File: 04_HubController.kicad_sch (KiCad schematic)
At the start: 1 part, among them U13 CYUSB3304-68LTXx

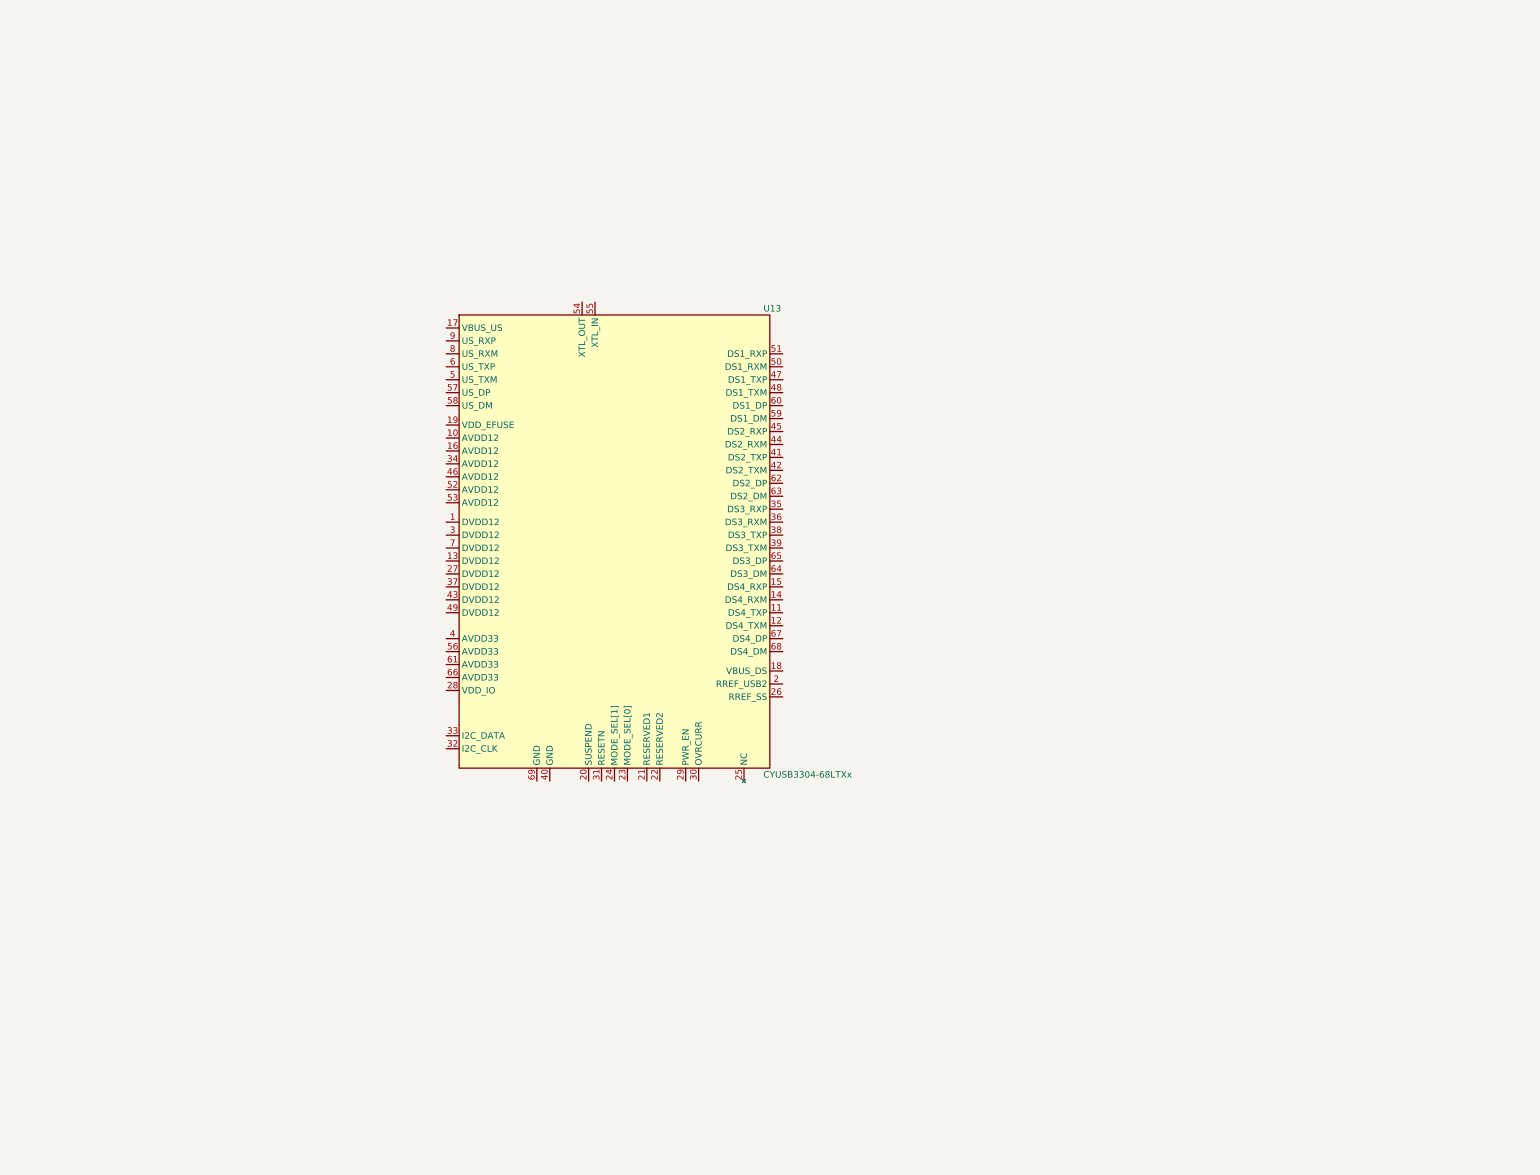
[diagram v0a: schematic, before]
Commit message: WIP hub and DFP
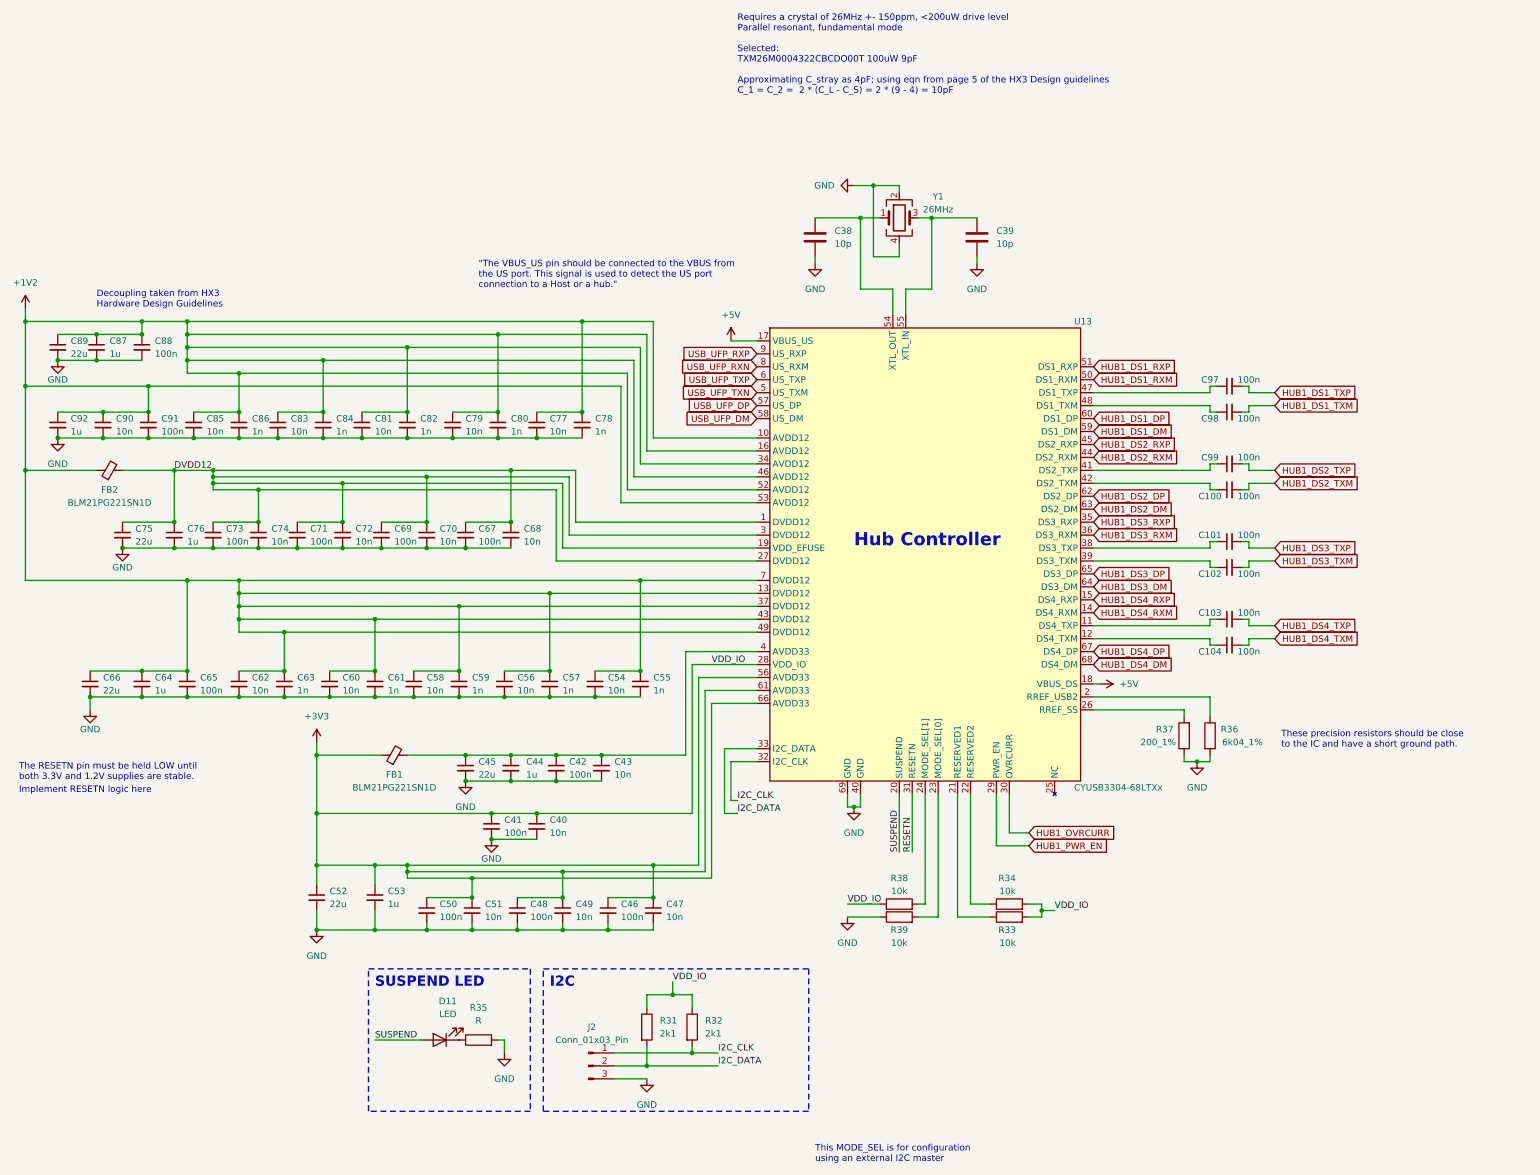
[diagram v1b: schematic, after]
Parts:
- added C100, C101, C102, C103, C104, C41, C42, C46, C48, C50, C65, C67, C69, C71, C73, C88, C91, C97, C98, C99: 100n, symbol Device:C_Small
- added C38, C39: 10p, symbol Device:C
- added C40, C43, C47, C49, C51, C54, C56, C58, C60, C62, C68, C70, C72, C74, C77, C79, C81, C83, C85, C90: 10n, symbol Device:C_Small
- added C44, C53, C64, C76, C87, C92: 1u, symbol Device:C_Small
- added C45, C52, C66, C75, C89: 22u, symbol Device:C_Small
- added C55, C57, C59, C61, C63, C78, C80, C82, C84, C86: 1n, symbol Device:C_Small
- added D11: LED, symbol Device:LED
- added FB1, FB2: BLM21PG221SN1D, symbol Device:FerriteBead_Small
- added J2: Conn_01x03_Pin, symbol Connector:Conn_01x03_Pin
- added R31, R32: 2k1, symbol Device:R
- added R33, R34, R38, R39: 10k, symbol Device:R
- added R35: R, symbol Device:R
- added R36: 6k04_1%, symbol Device:R
- added R37: 200_1%, symbol Device:R
- added Y1: 26MHz, symbol Device:Crystal_GND24
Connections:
- net DVDD12: now reaches U13.1 (DVDD12)
- net DVDD12: now also U13.19 (VDD_EFUSE), U13.27 (DVDD12), U13.3 (DVDD12), C67.1, C68.1, C69.1, C70.1, C71.1, C72.1, C73.1, C74.1, C75.1, C76.1, FB2.2
- net +1V2: now reaches U13.10 (AVDD12)
- net +1V2: now also U13.13 (DVDD12), U13.16 (AVDD12), U13.34 (AVDD12), U13.37 (DVDD12), U13.43 (DVDD12), U13.46 (AVDD12), U13.49 (DVDD12), U13.52 (AVDD12), U13.53 (AVDD12), U13.7 (DVDD12), C54.1, C55.1, C56.1, C57.1, C58.1, C59.1, C60.1, C61.1, C62.1, C63.1, C64.1, C65.1, C66.1, C77.1, C78.1, C79.1, C80.1, C81.1, C82.1, C83.1, C84.1, C85.1, C86.1, C87.1, C88.1, C89.1, C90.1, C91.1, C92.1, FB2.1
- net at U13.11 (DS4_TXP): now also C103.1
- net at U13.12 (DS4_TXM): now also C104.1
- net HUB1_DS4_RXM: now reaches U13.14 (DS4_RXM)
- net HUB1_DS4_RXP: now reaches U13.15 (DS4_RXP)
- net +5V: now reaches U13.17 (VBUS_US)
- net +5V: now also U13.18 (VBUS_DS)
- net at U13.2 (RREF_USB2): now also R36.1
- net SUSPEND: now reaches U13.20 (SUSPEND)
- net SUSPEND: now also D11.2 (A)
- net at U13.21 (RESERVED1): now also R33.1
- net at U13.22 (RESERVED2): now also R34.1
- net at U13.23 (MODE_SEL[0]): now also R39.2
- net at U13.24 (MODE_SEL[1]): now also R38.2
- net at U13.26 (RREF_SS): now also R37.2
- net +3V3: now reaches U13.28 (VDD_IO)
- net +3V3: now also U13.56 (AVDD33), U13.61 (AVDD33), U13.66 (AVDD33), C40.1, C41.1, C46.1, C47.1, C48.1, C49.1, C50.1, C51.1, C52.1, C53.1, FB1.1, R31.1, R32.1, R33.2, R34.2, R38.1
- net HUB1_PWR_EN: now reaches U13.29 (PWR_EN)
- net HUB1_OVRCURR: now reaches U13.30 (OVRCURR)
- net RESETN: now reaches U13.31 (RESETN)
- net I2C_CLK: now reaches U13.32 (I2C_CLK)
- net I2C_CLK: now also J2.1 (Pin_1), R32.2
- net I2C_DATA: now reaches U13.33 (I2C_DATA)
- net I2C_DATA: now also J2.2 (Pin_2), R31.2
- net HUB1_DS3_RXP: now reaches U13.35 (DS3_RXP)
- net HUB1_DS3_RXM: now reaches U13.36 (DS3_RXM)
- net at U13.38 (DS3_TXP): now also C101.1
- net at U13.39 (DS3_TXM): now also C102.1
- net at U13.4 (AVDD33): now also C42.1, C43.1, C44.1, C45.1, FB1.2
- net GND: now reaches U13.40 (GND)
- net GND: now also U13.69 (GND), C38.2, C39.2, C40.2, C41.2, C42.2, C43.2, C44.2, C45.2, C46.2, C47.2, C48.2, C49.2, C50.2, C51.2, C52.2, C53.2, C54.2, C55.2, C56.2, C57.2, C58.2, C59.2, C60.2, C61.2, C62.2, C63.2, C64.2, C65.2, C66.2, C67.2, C68.2, C69.2, C70.2, C71.2, C72.2, C73.2, C74.2, C75.2, C76.2, C77.2, C78.2, C79.2, C80.2, C81.2, C82.2, C83.2, C84.2, C85.2, C86.2, C87.2, C88.2, C89.2, C90.2, C91.2, C92.2, J2.3 (Pin_3), R35.2, R36.2, R37.1, R39.1, Y1.2, Y1.4
- net at U13.41 (DS2_TXP): now also C99.1
- net at U13.42 (DS2_TXM): now also C100.1
- net HUB1_DS2_RXM: now reaches U13.44 (DS2_RXM)
- net HUB1_DS2_RXP: now reaches U13.45 (DS2_RXP)
- net at U13.47 (DS1_TXP): now also C97.1
- net at U13.48 (DS1_TXM): now also C98.1
- net USB_UFP_TXN: now reaches U13.5 (US_TXM)
- net HUB1_DS1_RXM: now reaches U13.50 (DS1_RXM)
- net HUB1_DS1_RXP: now reaches U13.51 (DS1_RXP)
- net at U13.54 (XTL_OUT): now also C38.1, Y1.1
- net at U13.55 (XTL_IN): now also C39.1, Y1.3
- net USB_UFP_DP: now reaches U13.57 (US_DP)
- net USB_UFP_DM: now reaches U13.58 (US_DM)
- net HUB1_DS1_DM: now reaches U13.59 (DS1_DM)
- net USB_UFP_TXP: now reaches U13.6 (US_TXP)
- net HUB1_DS1_DP: now reaches U13.60 (DS1_DP)
- net HUB1_DS2_DP: now reaches U13.62 (DS2_DP)
- net HUB1_DS2_DM: now reaches U13.63 (DS2_DM)
- net HUB1_DS3_DM: now reaches U13.64 (DS3_DM)
- net HUB1_DS3_DP: now reaches U13.65 (DS3_DP)
- net HUB1_DS4_DP: now reaches U13.67 (DS4_DP)
- net HUB1_DS4_DM: now reaches U13.68 (DS4_DM)
- net USB_UFP_RXN: now reaches U13.8 (US_RXM)
- net USB_UFP_RXP: now reaches U13.9 (US_RXP)
- new net: D11.1 (K), R35.1
- new net HUB1_DS1_TXM: C98.2
- new net HUB1_DS1_TXP: C97.2
- new net HUB1_DS2_TXM: C100.2
- new net HUB1_DS2_TXP: C99.2
- new net HUB1_DS3_TXM: C102.2
- new net HUB1_DS3_TXP: C101.2
- new net HUB1_DS4_TXM: C104.2
- new net HUB1_DS4_TXP: C103.2
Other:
- note added: ""The VBUS_US pin should be connected to the VBUS from the US port. This signal is used to detect the US port connection to a Host or a hub.""
- note added: "Decoupling taken from HX3 Hardware Design Guidelines"
- note added: "Hub Controller"
- note added: "I2C"
- note added: "Implement RESETN logic here"
- note added: "Requires a crystal of 26MHz +- 150ppm, <200uW drive level Parallel resonant, fundamental mode Selected: TXM26M0004322CBCDO00T 100uW 9pF Approximating C_stray as 4pF; using eqn from page 5 of the HX3 Design guidelines C_1 = C_2 = 2 * (C_L - C_S) = 2 * (9 - 4) = 10pF"
- note added: "SUSPEND LED"
- note added: "The RESETN pin must be held LOW until both 3.3V and 1.2V supplies are stable."
- note added: "These precision resistors should be close to the IC and have a short ground path."
- note added: "This MODE_SEL is for configuration using an external I2C master"
- moved on the sheet: U13
